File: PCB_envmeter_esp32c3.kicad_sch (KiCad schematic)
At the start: 26 parts, among them J1 USB_C_Receptacle_USB2.0_16P, J2 USB_C_Receptacle_Simple, J3 AE-BME680, J4 SSD1306, SW1 Reset, SW2 Mode, U1 ESP32-C3-WROOM-02, U2 AP7333-33SAG, U3 NJM2845DL1-33

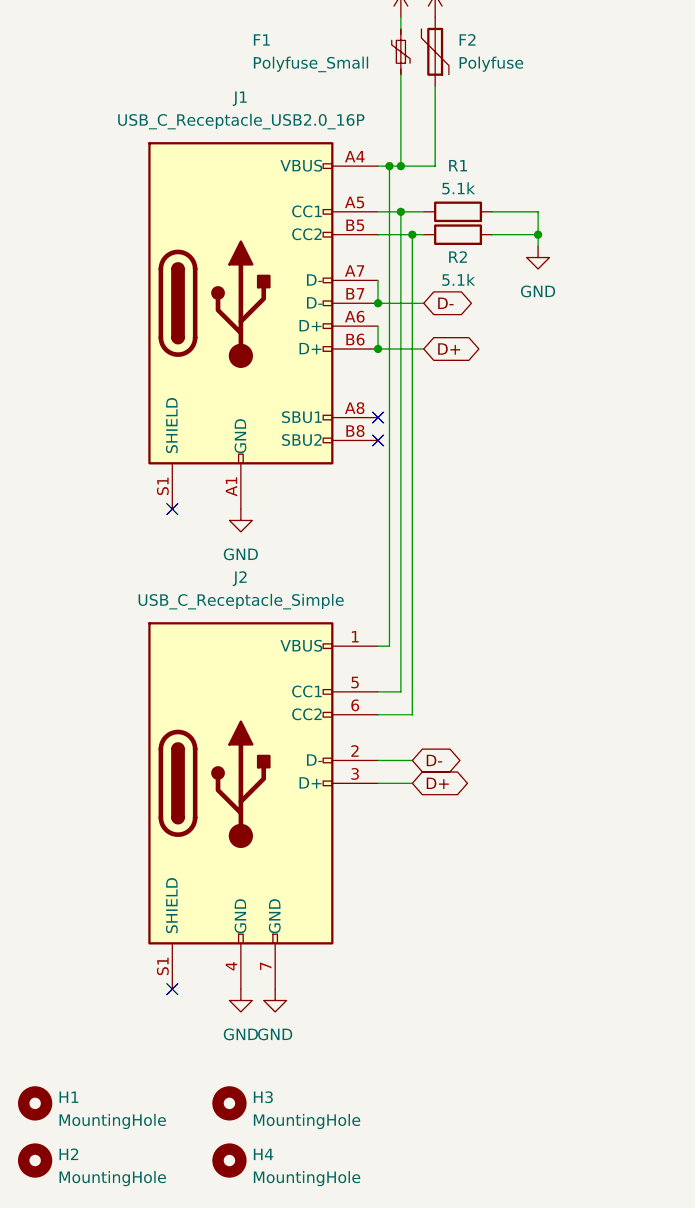
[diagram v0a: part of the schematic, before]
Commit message: Change footprint
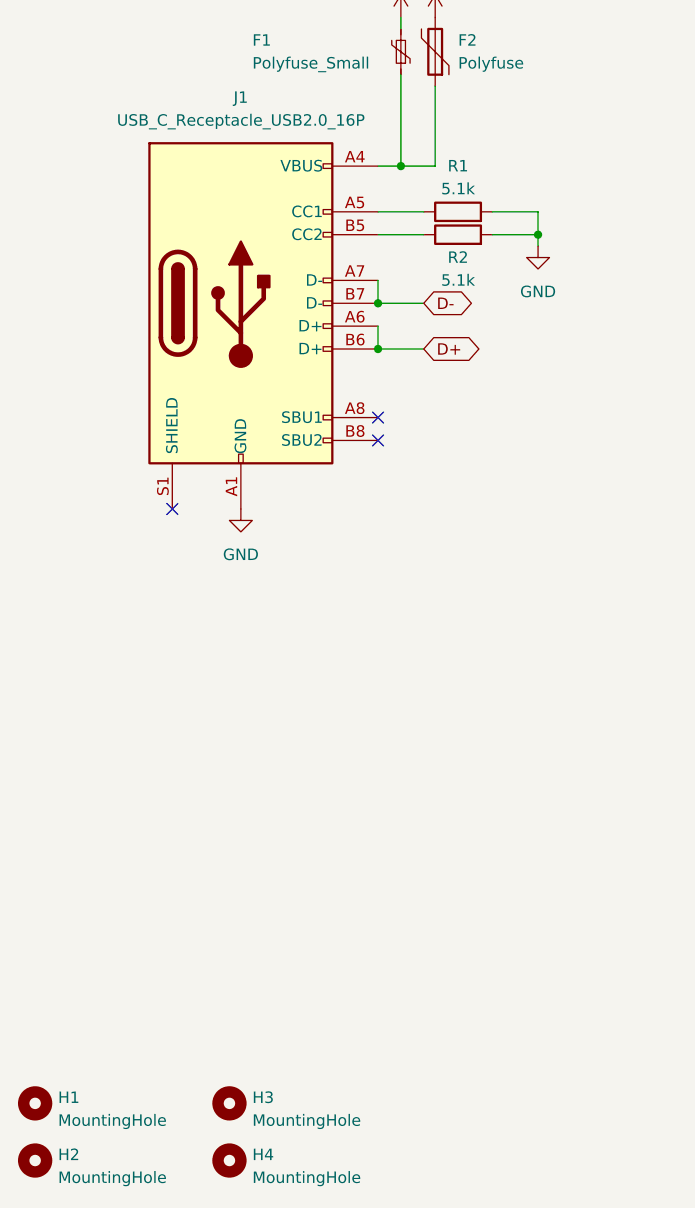
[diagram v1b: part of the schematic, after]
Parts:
- removed J2: USB_C_Receptacle_Simple, mylib:Connector_USB_C_simple, symbol mylib:USB_C_Receptacle_Simple
- J1: footprint Connector_USB:USB_C_Receptacle_XKB_U262-16XN-4BVC11 -> mylib:Connector_USB_C_simple_combo
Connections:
- no-connect marks 13 -> 12
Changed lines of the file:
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@@
   (junction (at 66.04 22.86) (diameter 0) (color 0 0 0 0)
-  )
-  (junction (at 59.69 86.36) (diameter 0) (color 0 0 0 0)
-  )
-  (junction (at 58.42 81.28) (diameter 0) (color 0 0 0 0)
-  )
-  (junction (at 60.96 88.9) (diameter 0) (color 0 0 0 0)
   )
   (junction (at 104.14 45.72) (diameter 0) (color 0 0 0 0)
@@
   (no_connect (at 200.66 115.57))
   (no_connect (at 200.66 82.55))
-  (no_connect (at 34.29 172.72))
   (no_connect (at 200.66 105.41))
   (no_connect (at 144.78 87.63))
@@
     (stroke (width 0) (type default))
   )
-  (wire (pts (xy 57.15 81.28) (xy 58.42 81.28))
+  (wire (pts (xy 57.15 81.28) (xy 59.69 81.28))
     (stroke (width 0) (type default))
   )
@@
     (stroke (width 0) (type default))
   )
-  (wire (pts (xy 60.96 142.24) (xy 60.96 88.9))
-    (stroke (width 0) (type default))
-  )
   (wire (pts (xy 59.69 81.28) (xy 59.69 71.12))
     (stroke (width 0) (type default))
   )
-  (wire (pts (xy 62.23 88.9) (xy 60.96 88.9))
-    (stroke (width 0) (type default))
-  )
   (wire (pts (xy 63.5 72.39) (xy 63.5 81.28))
     (stroke (width 0) (type default))
@@
     (stroke (width 0) (type default))
   )
-  (wire (pts (xy 57.15 142.24) (xy 60.96 142.24))
-    (stroke (width 0) (type default))
-  )
   (wire (pts (xy 111.76 143.51) (xy 114.3 143.51))
     (stroke (width 0) (type default))
@@
     (stroke (width 0) (type default))
   )
-  (wire (pts (xy 60.96 147.32) (xy 57.15 147.32))
-    (stroke (width 0) (type default))
-  )
-  (wire (pts (xy 57.15 134.62) (xy 58.42 134.62))
-    (stroke (width 0) (type default))
-  )
   (wire (pts (xy 200.66 102.87) (xy 227.33 102.87))
     (stroke (width 0) (type default))
@@
     (stroke (width 0) (type default))
   )
-  (wire (pts (xy 59.69 86.36) (xy 57.15 86.36))
-    (stroke (width 0) (type default))
-  )
-  (wire (pts (xy 58.42 81.28) (xy 59.69 81.28))
+  (wire (pts (xy 57.15 86.36) (xy 62.23 86.36))
     (stroke (width 0) (type default))
   )
@@
     (stroke (width 0) (type default))
   )
-  (wire (pts (xy 62.23 86.36) (xy 59.69 86.36))
-    (stroke (width 0) (type default))
-  )
   (wire (pts (xy 74.93 90.17) (xy 74.93 88.9))
     (stroke (width 0) (type default))
   )
-  (wire (pts (xy 60.96 149.86) (xy 57.15 149.86))
-    (stroke (width 0) (type default))
-  )
   (wire (pts (xy 110.49 24.13) (xy 110.49 22.86))
     (stroke (width 0) (type default))
@@
     (stroke (width 0) (type default))
   )
-  (wire (pts (xy 58.42 134.62) (xy 58.42 81.28))
-    (stroke (width 0) (type default))
-  )
   (wire (pts (xy 110.49 29.21) (xy 110.49 30.48))
     (stroke (width 0) (type default))
@@
     (stroke (width 0) (type default))
   )
-  (wire (pts (xy 60.96 88.9) (xy 57.15 88.9))
+  (wire (pts (xy 57.15 88.9) (xy 62.23 88.9))
     (stroke (width 0) (type default))
   )
@@
     (stroke (width 0) (type default))
   )
-  (wire (pts (xy 59.69 139.7) (xy 59.69 86.36))
-    (stroke (width 0) (type default))
-  )
   (wire (pts (xy 111.76 170.18) (xy 114.3 170.18))
     (stroke (width 0) (type default))
@@
   )
   (wire (pts (xy 63.5 81.28) (xy 59.69 81.28))
-    (stroke (width 0) (type default))
-  )
-  (wire (pts (xy 57.15 139.7) (xy 59.69 139.7))
     (stroke (width 0) (type default))
   )
@@
     (effects (font (size 1.27 1.27)) (justify left))
     (property "Intersheetrefs" "${INTERSHEET_REFS}" (at 243.8241 102.87 0)
-      (effects (font (size 1.27 1.27)) (justify left) hide)
-    )
-  )
-  (global_label "D+" (shape bidirectional) (at 60.96 149.86 0) (fields_autoplaced)
-    (effects (font (size 1.27 1.27)) (justify left))
-    (property "Intersheetrefs" "${INTERSHEET_REFS}" (at 67.8989 149.86 0)
-      (effects (font (size 1.27 1.27)) (justify left) hide)
-    )
-  )
-  (global_label "D-" (shape bidirectional) (at 60.96 147.32 0) (fields_autoplaced)
-    (effects (font (size 1.27 1.27)) (justify left))
-    (property "Intersheetrefs" "${INTERSHEET_REFS}" (at 67.8989 147.32 0)
       (effects (font (size 1.27 1.27)) (justify left) hide)
     )
@@
     )
   )
-  (symbol (lib_id "power:GND") (at 41.91 172.72 0) (unit 1)
-    (in_bom yes) (on_board yes) (dnp no) (fields_autoplaced)
-    (property "Reference" "#PWR027" (at 41.91 179.07 0)
-      (effects (font (size 1.27 1.27)) hide)
-    )
-    (property "Value" "GND" (at 41.91 177.8 0)
-      (effects (font (size 1.27 1.27)))
-    )
-    (property "Footprint" "" (at 41.91 172.72 0)
-      (effects (font (size 1.27 1.27)) hide)
-    )
-    (property "Datasheet" "" (at 41.91 172.72 0)
-      (effects (font (size 1.27 1.27)) hide)
-    )
-    (pin "1")
-    (instances
-      (project "PCB_envmeter_esp32c3"
-        (path "/e56fcc30-bb74-4f59-a961-89b735db6e9b"
-          (reference "#PWR027") (unit 1)
-        )
-      )
-    )
-  )
   (symbol (lib_id "Connector:USB_C_Receptacle_USB2.0_16P") (at 41.91 96.52 0) (unit 1)
     (in_bom yes) (on_board yes) (dnp no) (fields_autoplaced)
@@
       (effects (font (size 1.27 1.27)))
     )
-    (property "Footprint" "Connector_USB:USB_C_Receptacle_XKB_U262-16XN-4BVC11" (at 45.72 96.52 0)
+    (property "Footprint" "mylib:Connector_USB_C_simple_combo" (at 45.72 96.52 0)
       (effects (font (size 1.27 1.27)) hide)
     )
@@
     )
   )
-  (symbol (lib_id "mylib:USB_C_Receptacle_Simple") (at 41.91 149.86 0) (unit 1)
-    (in_bom yes) (on_board yes) (dnp no) (fields_autoplaced)
-    (property "Reference" "J2" (at 41.91 127 0)
-      (effects (font (size 1.27 1.27)))
-    )
-    (property "Value" "USB_C_Receptacle_Simple" (at 41.91 129.54 0)
-      (effects (font (size 1.27 1.27)))
-    )
-    (property "Footprint" "mylib:Connector_USB_C_simple" (at 45.72 149.86 0)
-      (effects (font (size 1.27 1.27)) hide)
-    )
-    (property "Datasheet" "https://www.usb.org/sites/default/files/documents/usb_type-c.zip" (at 45.72 149.86 0)
-      (effects (font (size 1.27 1.27)) hide)
-    )
-    (pin "S1")
-    (pin "A9")
-    (pin "A12")
-    (pin "5")
-    (pin "B4")
-    (pin "B6")
-    (pin "B9")
-    (pin "B7")
-    (pin "1")
-    (pin "7")
-    (pin "2")
-    (pin "6")
-    (pin "B12")
-    (pin "3")
-    (pin "4")
-    (instances
-      (project "PCB_envmeter_esp32c3"
-        (path "/e56fcc30-bb74-4f59-a961-89b735db6e9b"
-          (reference "J2") (unit 1)
-        )
-      )
-    )
-  )
   (symbol (lib_id "power:+3.3V") (at 172.72 74.93 0) (unit 1)
     (in_bom yes) (on_board yes) (dnp no) (fields_autoplaced)
@@
         )
       )
-    )
-  )
-  (symbol (lib_id "power:GND") (at 45.72 172.72 0) (unit 1)
-    (in_bom yes) (on_board yes) (dnp no) (fields_autoplaced)
-    (property "Reference" "#PWR026" (at 45.72 179.07 0)
-      (effects (font (size 1.27 1.27)) hide)
-    )
-    (property "Value" "GND" (at 45.72 177.8 0)
-      (effects (font (size 1.27 1.27)))
-    )
-    (property "Footprint" "" (at 45.72 172.72 0)
-      (effects (font (size 1.27 1.27)) hide)
-    )
-    (property "Datasheet" "" (at 45.72 172.72 0)
-      (effects (font (size 1.27 1.27)) hide)
-    )
-    (pin "1")
-    (instances
-      (project "PCB_envmeter_esp32c3"
-        (path "/e56fcc30-bb74-4f59-a961-89b735db6e9b"
-          (reference "#PWR026") (unit 1)
-        )
-      )

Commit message: Update F1 footprint
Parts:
- F1: footprint Capacitor_SMD:C_1210_3225Metric_Pad1.33x2.70mm_HandSolder -> Fuse:Fuse_1206_3216Metric_Pad1.42x1.75mm_HandSolder
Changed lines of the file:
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@@
       (effects (font (size 1.27 1.27)) (justify right))
     )
-    (property "Footprint" "Capacitor_SMD:C_1210_3225Metric_Pad1.33x2.70mm_HandSolder" (at 58.42 63.5 0)
+    (property "Footprint" "Fuse:Fuse_1206_3216Metric_Pad1.42x1.75mm_HandSolder" (at 58.42 63.5 0)
       (effects (font (size 1.27 1.27)) (justify left) hide)
     )
